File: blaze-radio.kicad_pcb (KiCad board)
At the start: 4 copper layers, 16 x 16 mm, 44 parts, among them J1 Conn_02x08_Castelated, J2 TagConnect_TC2030, U2 EFR32xG23xxxxF512xM48, U3 TSS-13HLN+, Y1 32.768KHz, Y2 38.400MHz

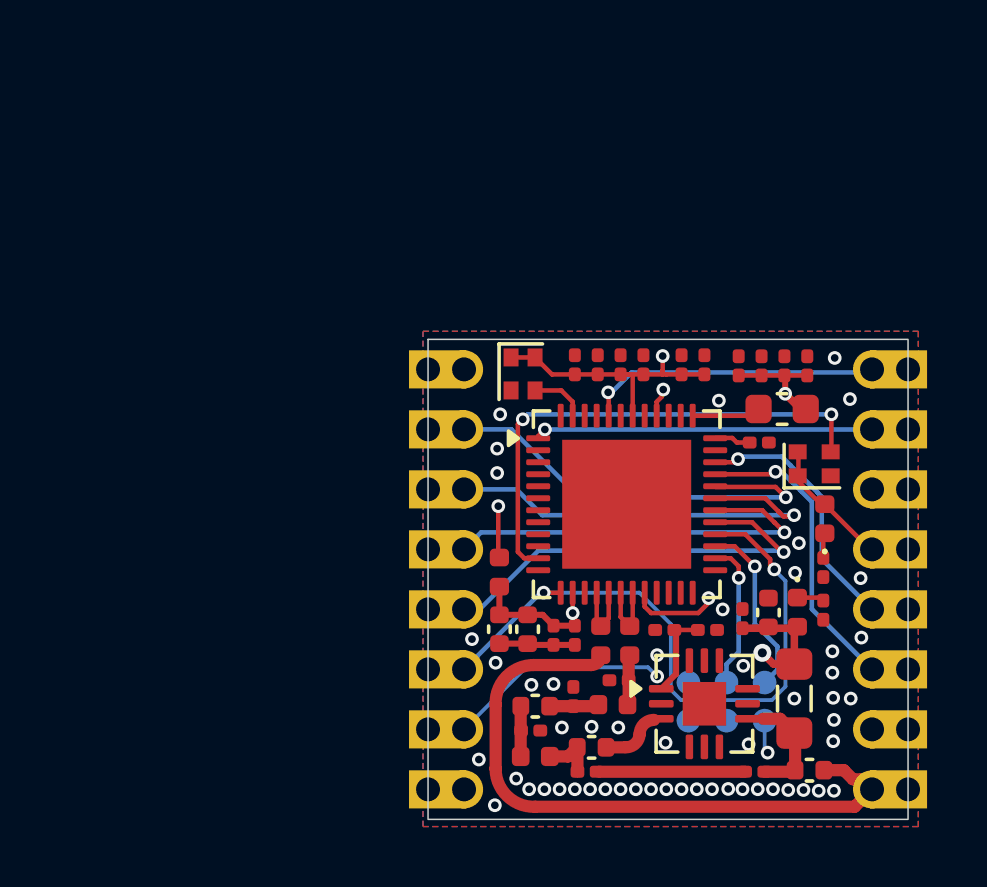
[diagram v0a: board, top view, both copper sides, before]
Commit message: Added git ignore
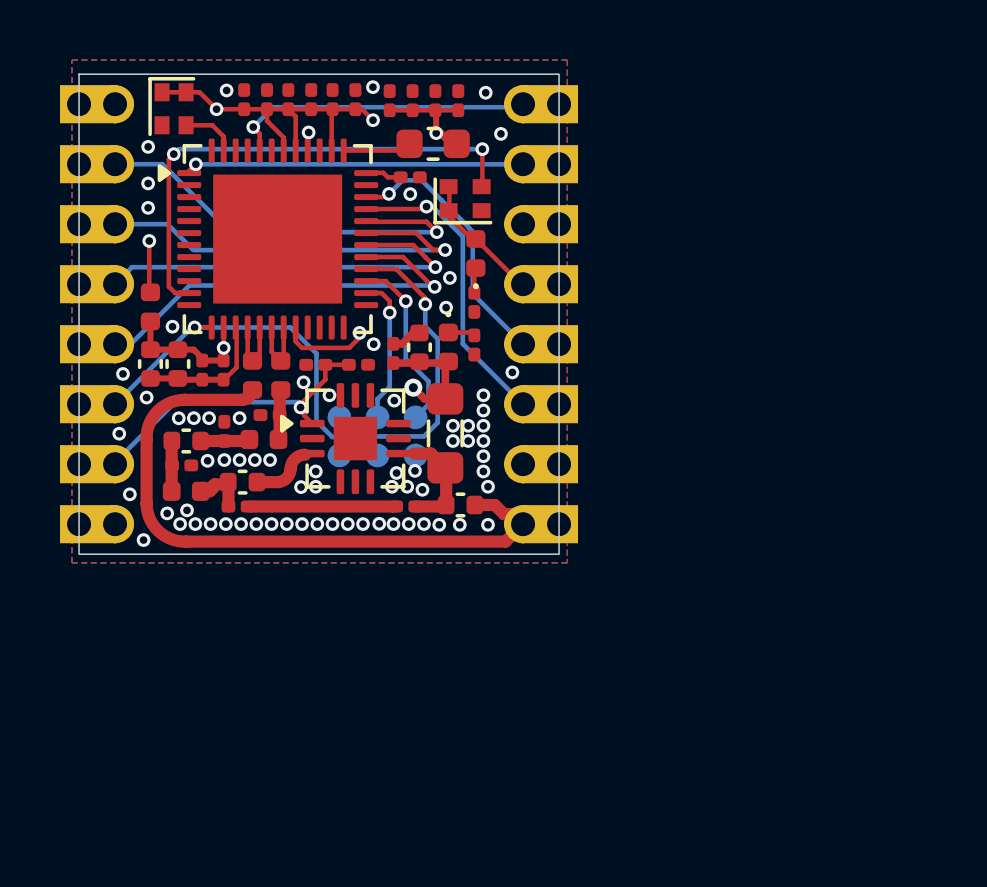
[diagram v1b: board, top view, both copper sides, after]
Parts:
- moved C16 14.7 mm to (102.4, 70.8)
- moved C17 14.7 mm to (103.1, 70.8)
- moved C15 14.6 mm to (101.6, 70.6)
- moved C18 14.6 mm to (101.9, 73.2)
- moved C19 14.6 mm to (104.6, 72.3)
- moved C20 14.6 mm to (103.1, 72.8)
- moved C23 14.6 mm to (103.6, 75.3)
- moved C24 14.6 mm to (109.6, 70.0)
- moved C25 14.6 mm to (106.2, 70.6)
- moved C26 14.6 mm to (108.8, 70.2)
- moved C29 14.6 mm to (101.7, 74.0)
- moved D1 14.6 mm to (111.5, 66.9)
- moved D2 14.6 mm to (110.6, 70.0)
- moved J2 14.6 mm to (108.2, 73.0)
- moved L6 14.6 mm to (110.5, 72.9)
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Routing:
- net GND: track 2.48 -> 5.44 mm, vias 53 -> 70
- net +3V3: track 14.0 -> 16.2 mm, vias 2 -> 3
- net VDD: track 11.8 -> 12.4 mm
